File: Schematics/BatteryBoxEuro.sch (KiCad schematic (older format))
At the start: 16 parts, among them K1 JD2912-1Z-12VDC_40A, P1 Conn_WallPlug, U2 F_Distributor, U3 NAC3MPA-1-WOT, U4 DPlusSimulator, U5 Pulser, U6 230V_KfzCharger, X1 X3, X2 12VKfz_Plug, X3 X3

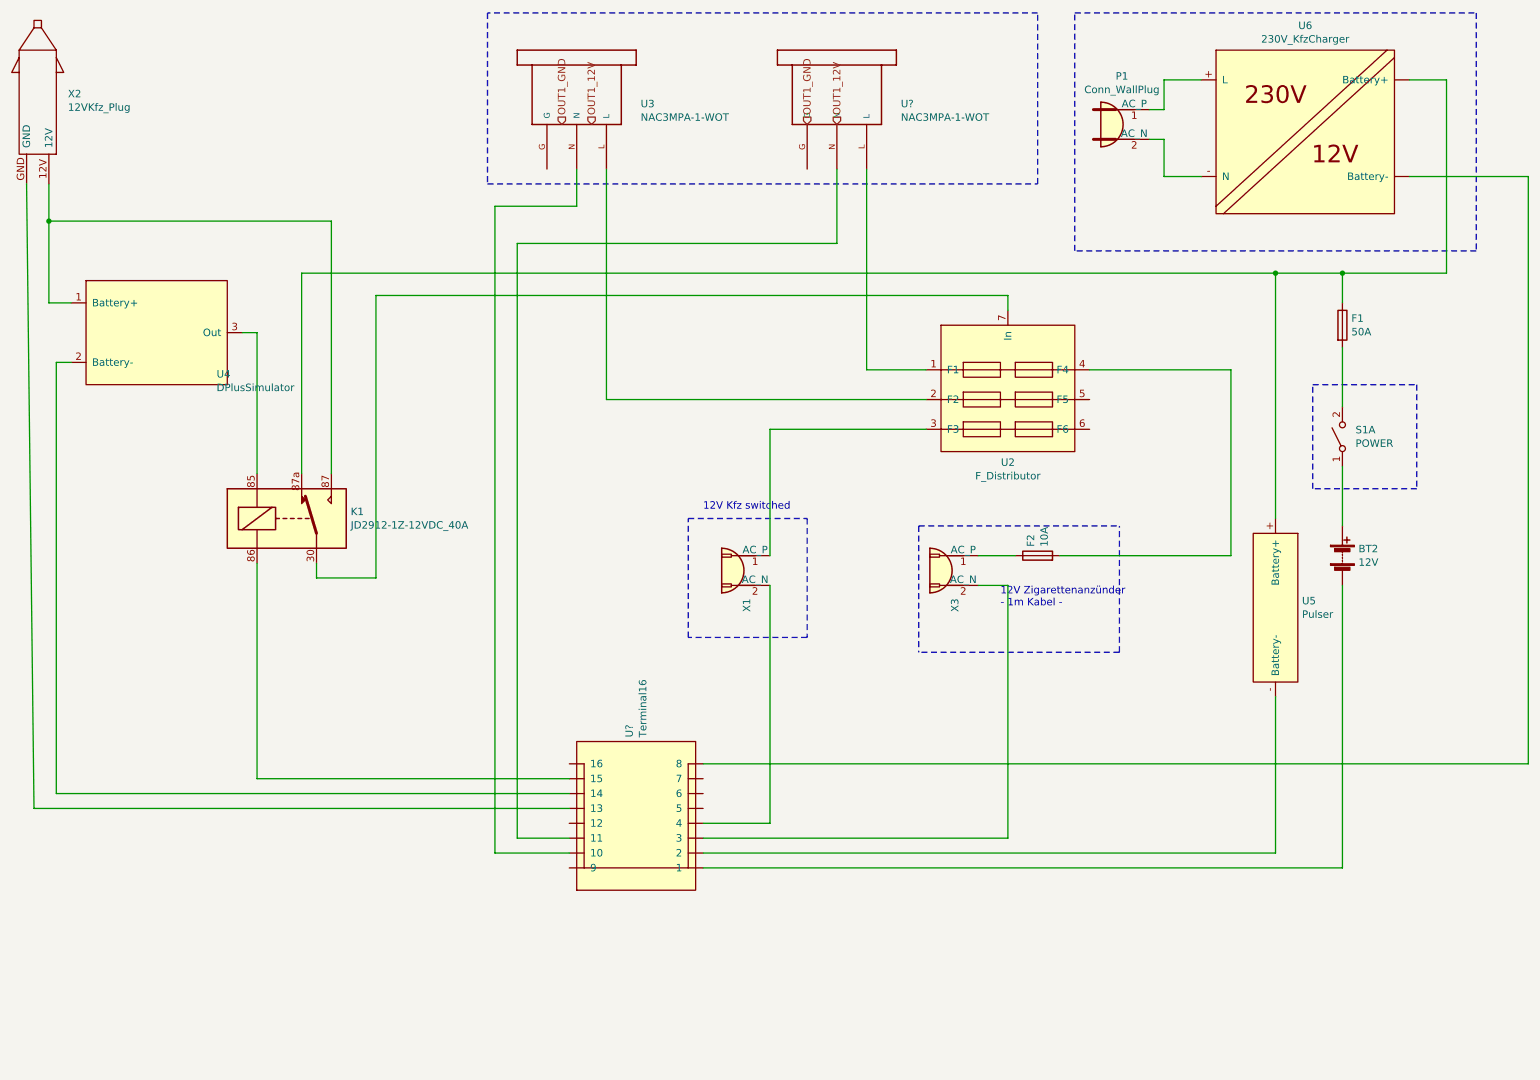
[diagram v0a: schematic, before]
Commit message: add filed
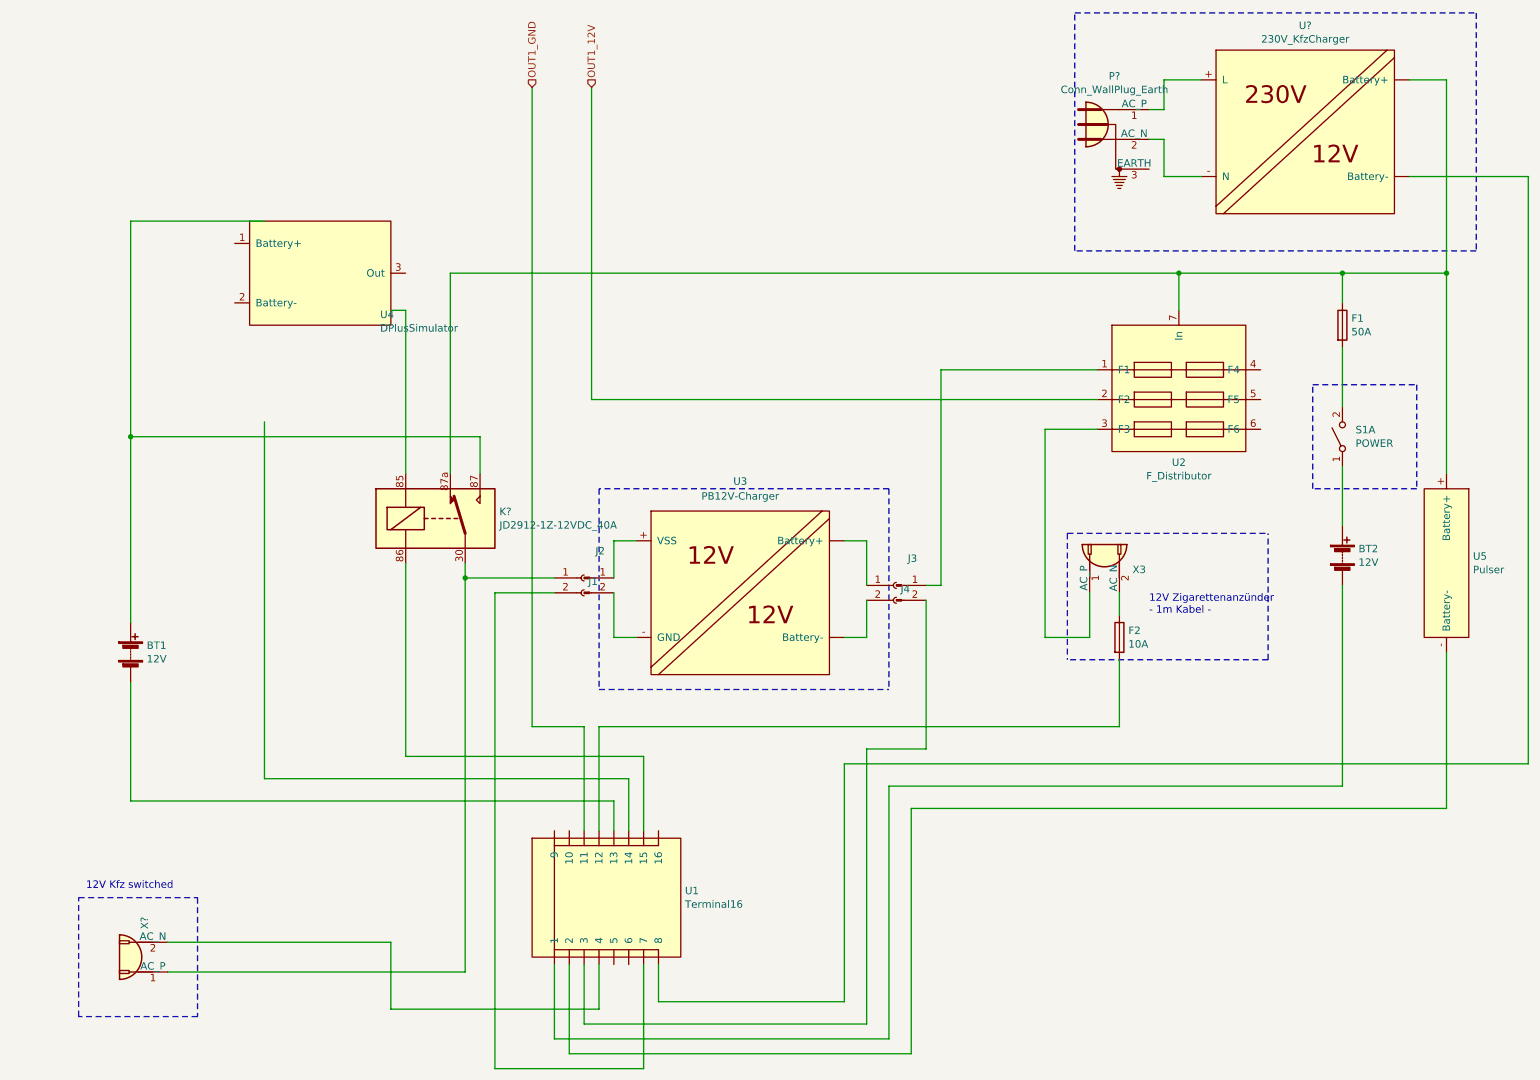
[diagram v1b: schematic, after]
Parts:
- removed P1: Conn_WallPlug, symbol Connector:Conn_WallPlug
- removed U3, U?: NAC3MPA-1-WOT, NAC3MPA-1-WOT, symbol NAC3MPA-1-WOT:NAC3MPA-1-WOT
- removed U?: Terminal16, symbol MyParts:Terminal16
- removed X2: 12VKfz_Plug, symbol MyParts:12VKfz_Plug
- added BT1: 12V, symbol Device:Battery
- added J1, J4: (no value), symbol Connector:Conn_01x02_Female
- added J2, J3: (no value), symbol Connector:Conn_01x02_Male
- added P?: Conn_WallPlug_Earth, symbol Connector:Conn_WallPlug_Earth
- added U1: Terminal16, symbol MyParts:Terminal16
- added U3: PB12V-Charger, symbol MyParts:PB12V-Charger
- renumbered K1 to K?, U6 to U?, X1 to X?
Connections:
- wire segments 65 -> 90
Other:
- moved on the sheet: F2, K?, U2, U4, U5, X3, X?
